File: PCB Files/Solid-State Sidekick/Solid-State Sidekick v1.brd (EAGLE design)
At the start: 66 x 72.4 mm, 6 parts, among them J1 C14, J2 NEMA, J3 RLY Control, SW1 Rocker

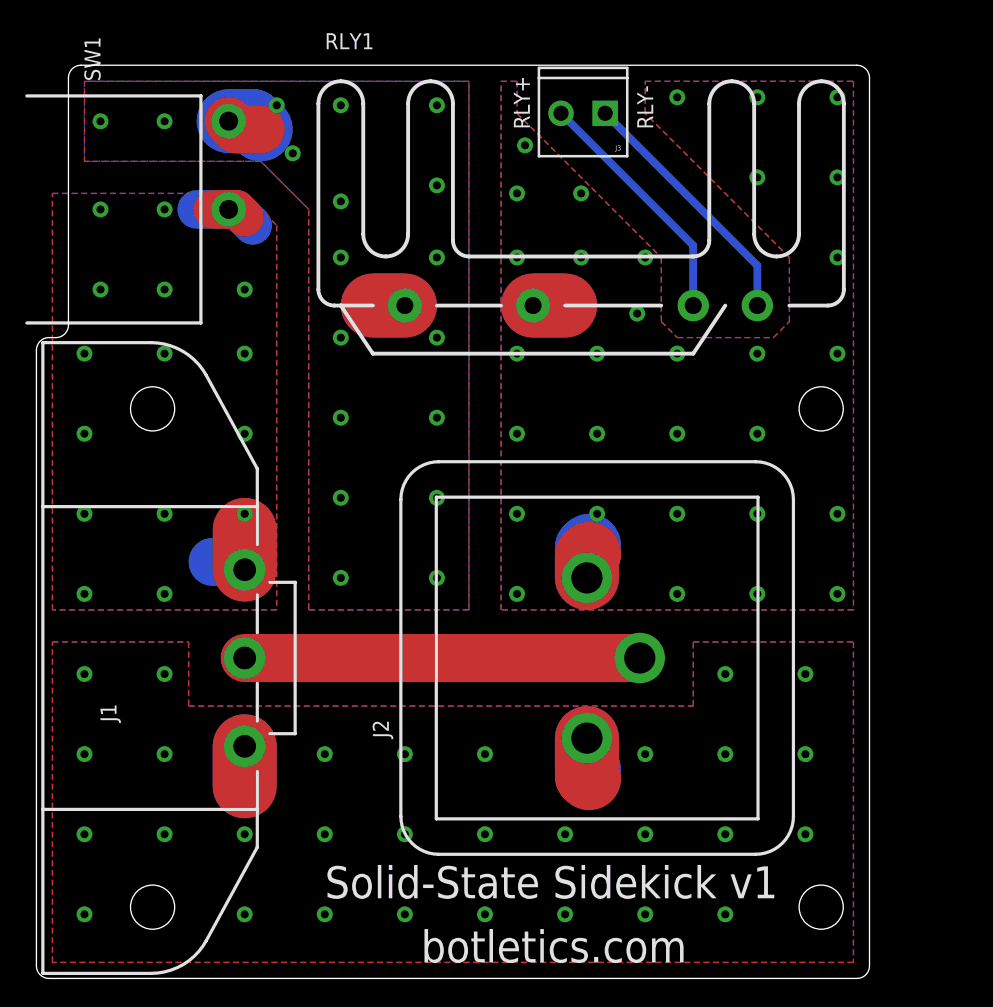
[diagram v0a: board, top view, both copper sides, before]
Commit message: Add files via upload
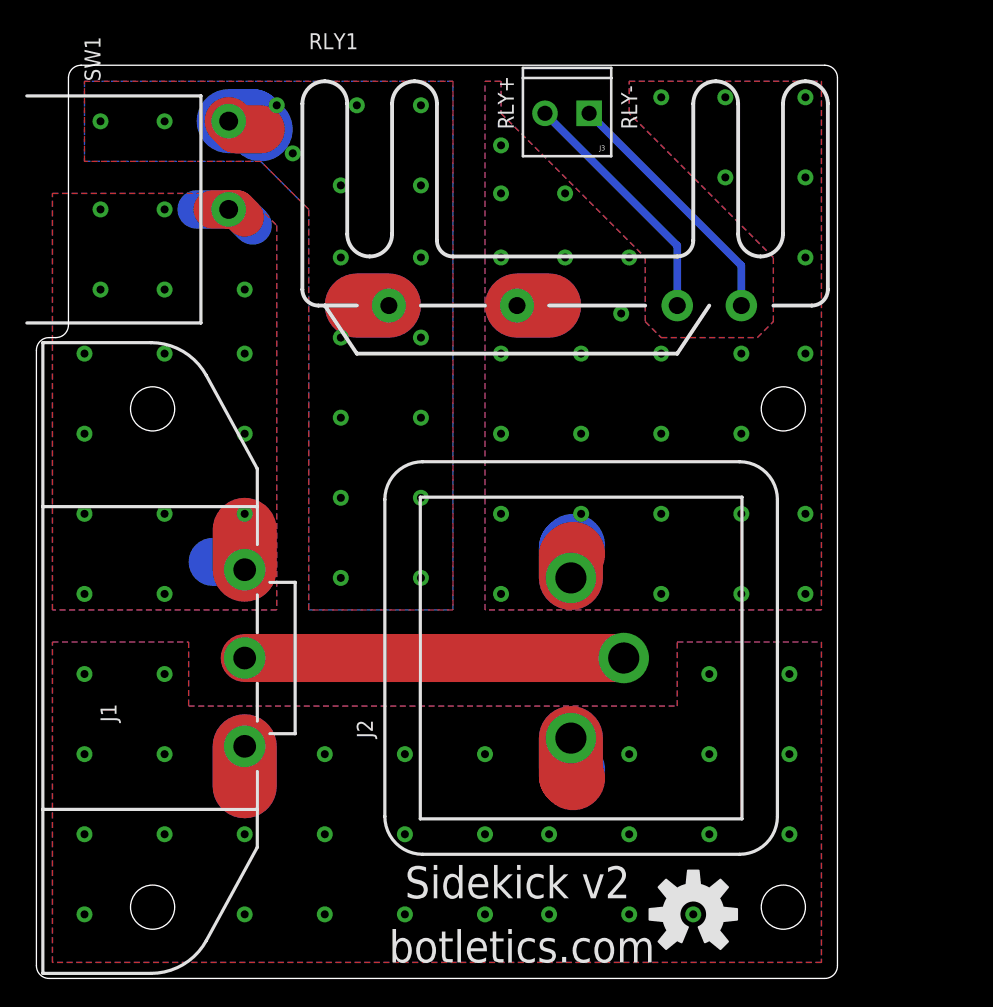
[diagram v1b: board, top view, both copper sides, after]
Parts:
- moved LOGO1 2.54 mm to (52.1, 5.08), flipped to the top
- moved J2 1.27 mm to (43.2, 25.4)
- moved J3 1.27 mm to (43.8, 68.6)
- moved RLY1 1.27 mm to (41.9, 53.3)
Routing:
- net GND: track 31.3 -> 30.1 mm
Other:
- board size 66 x 72.4 mm -> 63.5 x 72.4 mm
- board text added: "Sidekick v2"
- board text removed: "Solid-State Sidekick v1"
